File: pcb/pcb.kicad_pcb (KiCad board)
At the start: 2 copper layers, 18 x 10 mm, 1 part

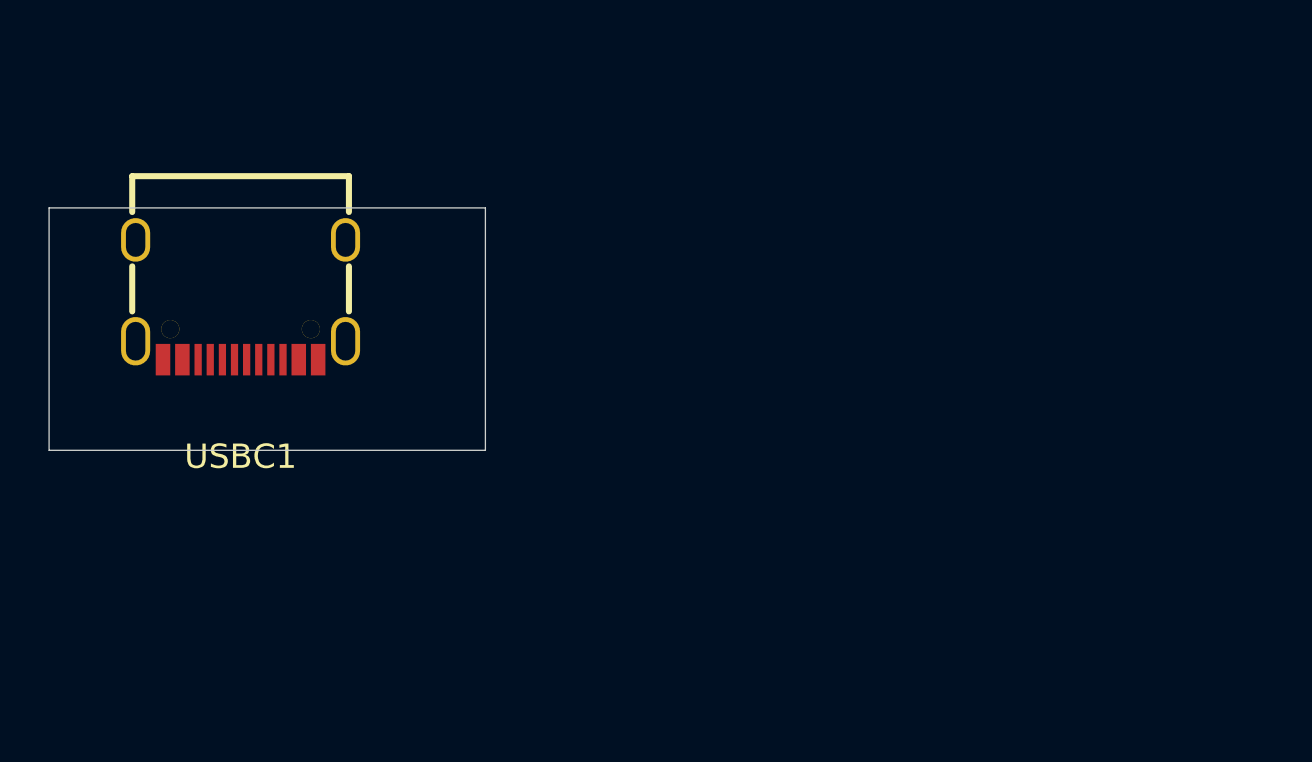
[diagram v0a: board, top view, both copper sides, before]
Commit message: More playing with JLCPCB
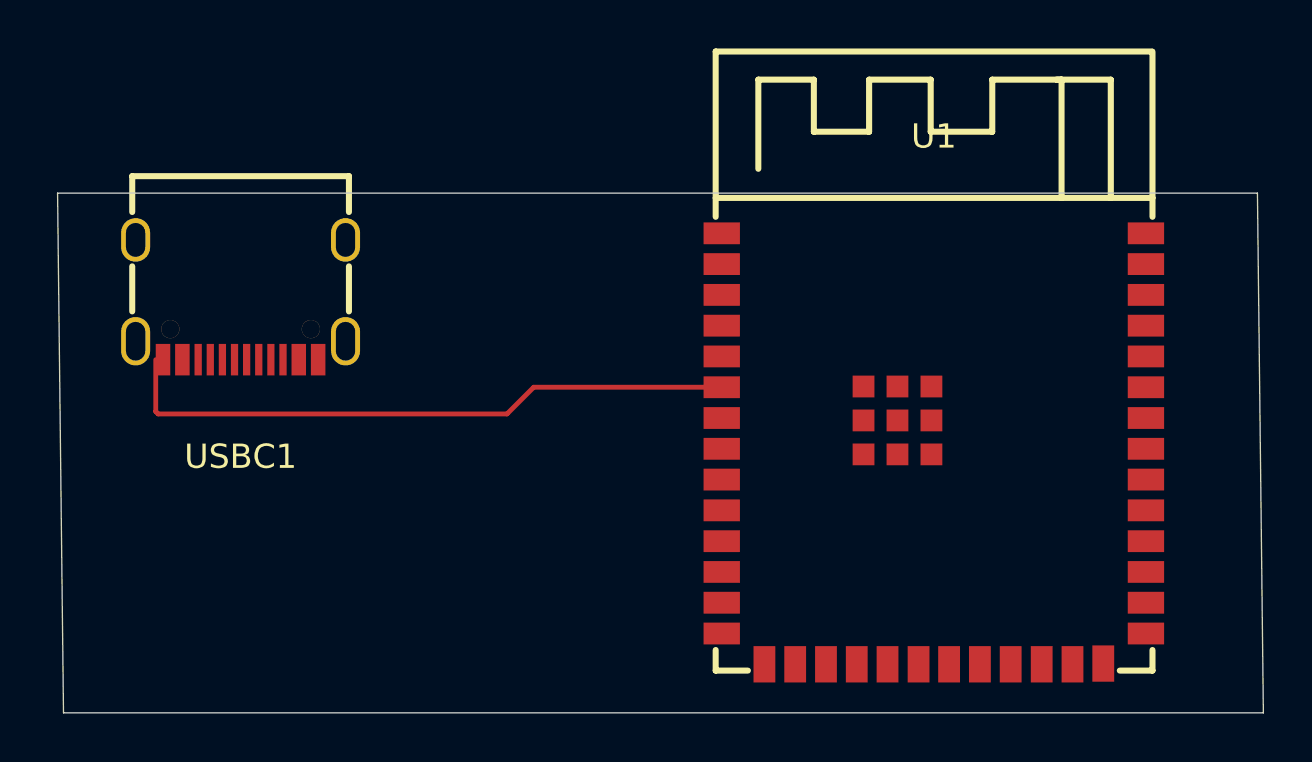
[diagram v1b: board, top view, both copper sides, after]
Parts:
- added U1: ESP32-S3-WROOM-1(N8R8), EasyEDA:WIRELM-SMD_ESP32-S3-WROOM-1, F.Cu at (186.0, 69.9)
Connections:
- USBC1 pad A12: unconnected-(USBC1-GND-PadA12) -> Net-(U1-IO6)
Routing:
- net Net-(U1-IO6): track 0.00 -> 26.0 mm
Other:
- board size 18 x 10 mm -> 49.7 x 21.4 mm
